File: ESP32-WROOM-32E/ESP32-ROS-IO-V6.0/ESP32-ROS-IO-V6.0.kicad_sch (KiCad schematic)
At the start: 2 parts, among them J1 Conn_01x22_Socket, J2 Conn_01x22_Socket

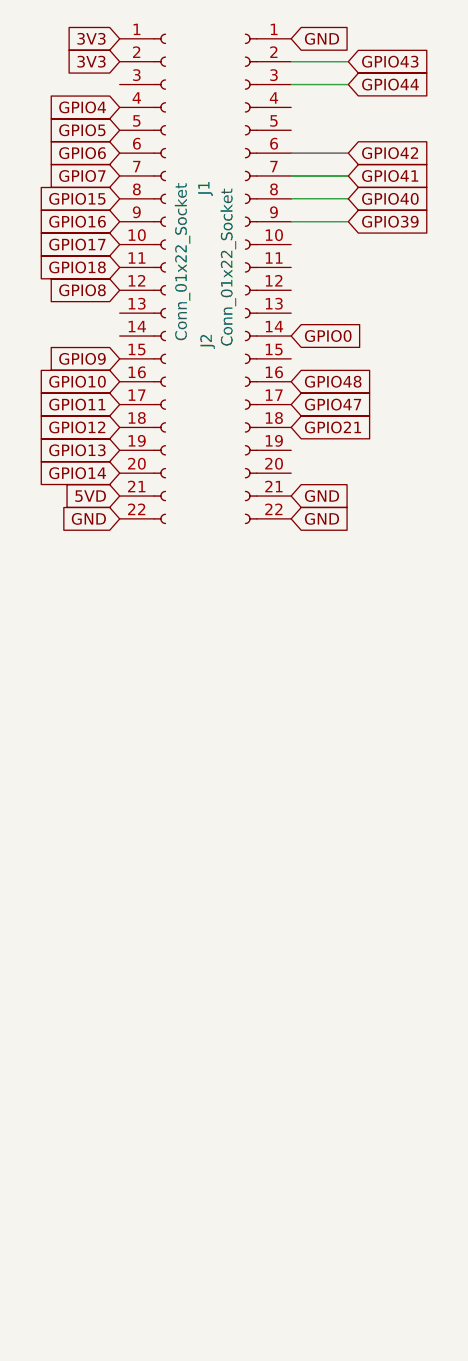
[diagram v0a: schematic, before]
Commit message: う
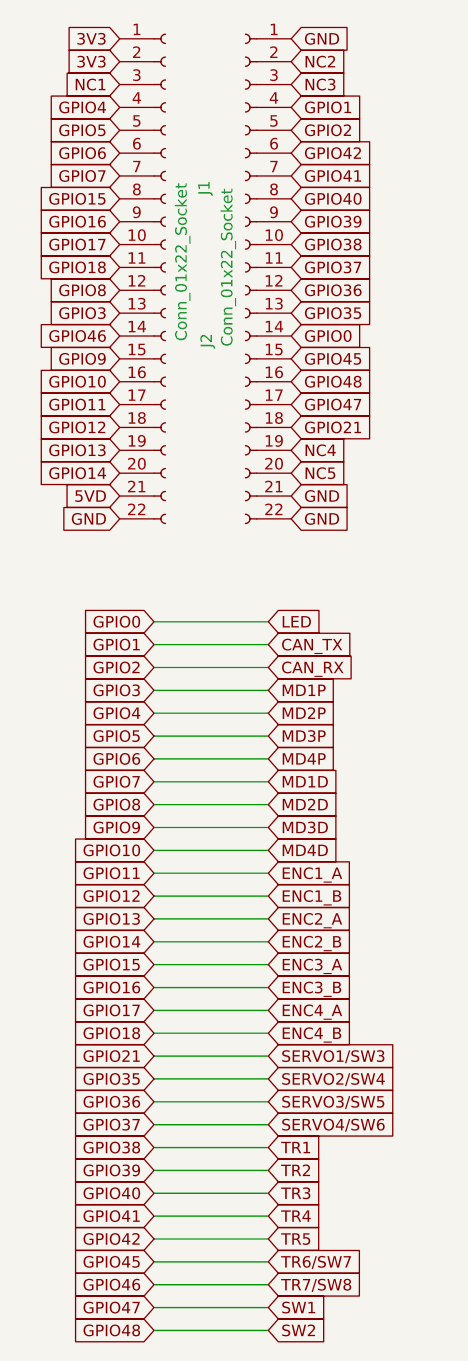
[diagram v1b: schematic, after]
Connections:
- net GPIO38: now reaches J2.10 (Pin_10)
- net GPIO37: now reaches J2.11 (Pin_11)
- net GPIO36: now reaches J2.12 (Pin_12)
- net GPIO35: now reaches J2.13 (Pin_13)
- net GPIO45: now reaches J2.15 (Pin_15)
- net NC4: now reaches J2.19 (Pin_19)
- net NC5: now reaches J2.20 (Pin_20)
- net CAN_TX: now reaches J2.4 (Pin_4)
- net CAN_RX: now reaches J2.5 (Pin_5)
- net GPIO3: now reaches J1.13 (Pin_13)
- net GPIO46: now reaches J1.14 (Pin_14)
- net NC1: now reaches J1.3 (Pin_3)
- net GPIO11 renamed ENC1_A
- net GPIO12 renamed ENC1_B
- net GPIO13 renamed ENC2_A
- net GPIO14 renamed ENC2_B
- net GPIO15 renamed ENC3_A
- net GPIO16 renamed ENC3_B
- net GPIO17 renamed ENC4_A
- net GPIO18 renamed ENC4_B
- net GPIO43 renamed NC2
- net GPIO44 renamed NC3

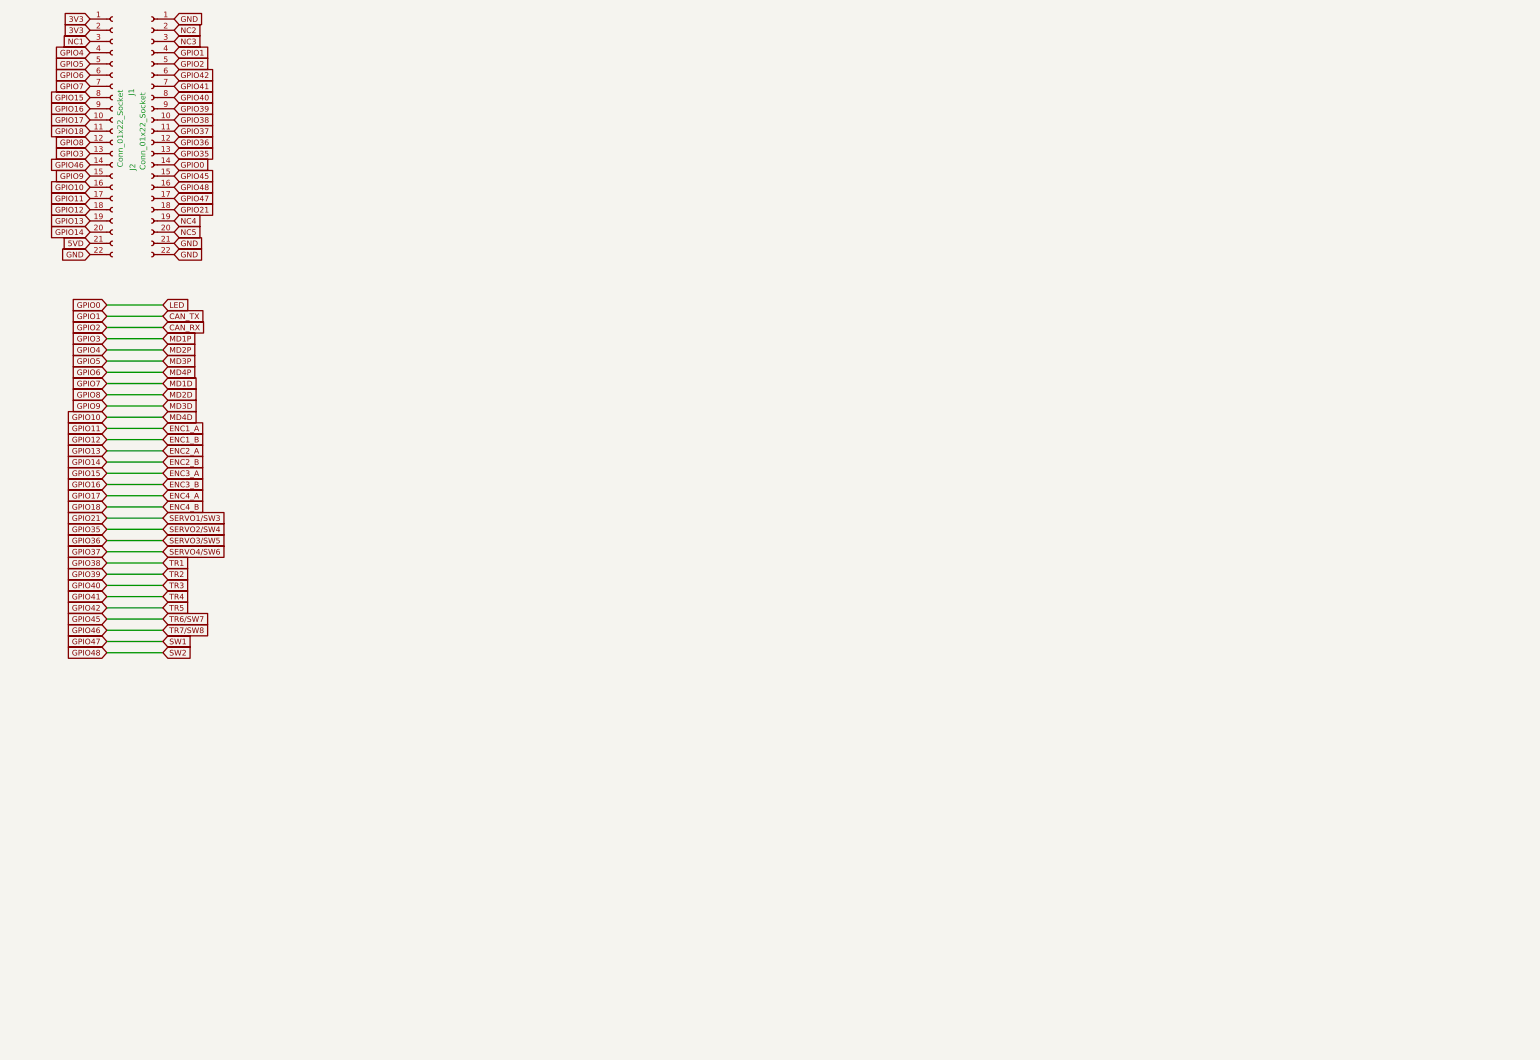
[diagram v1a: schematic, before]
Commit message: 回路図
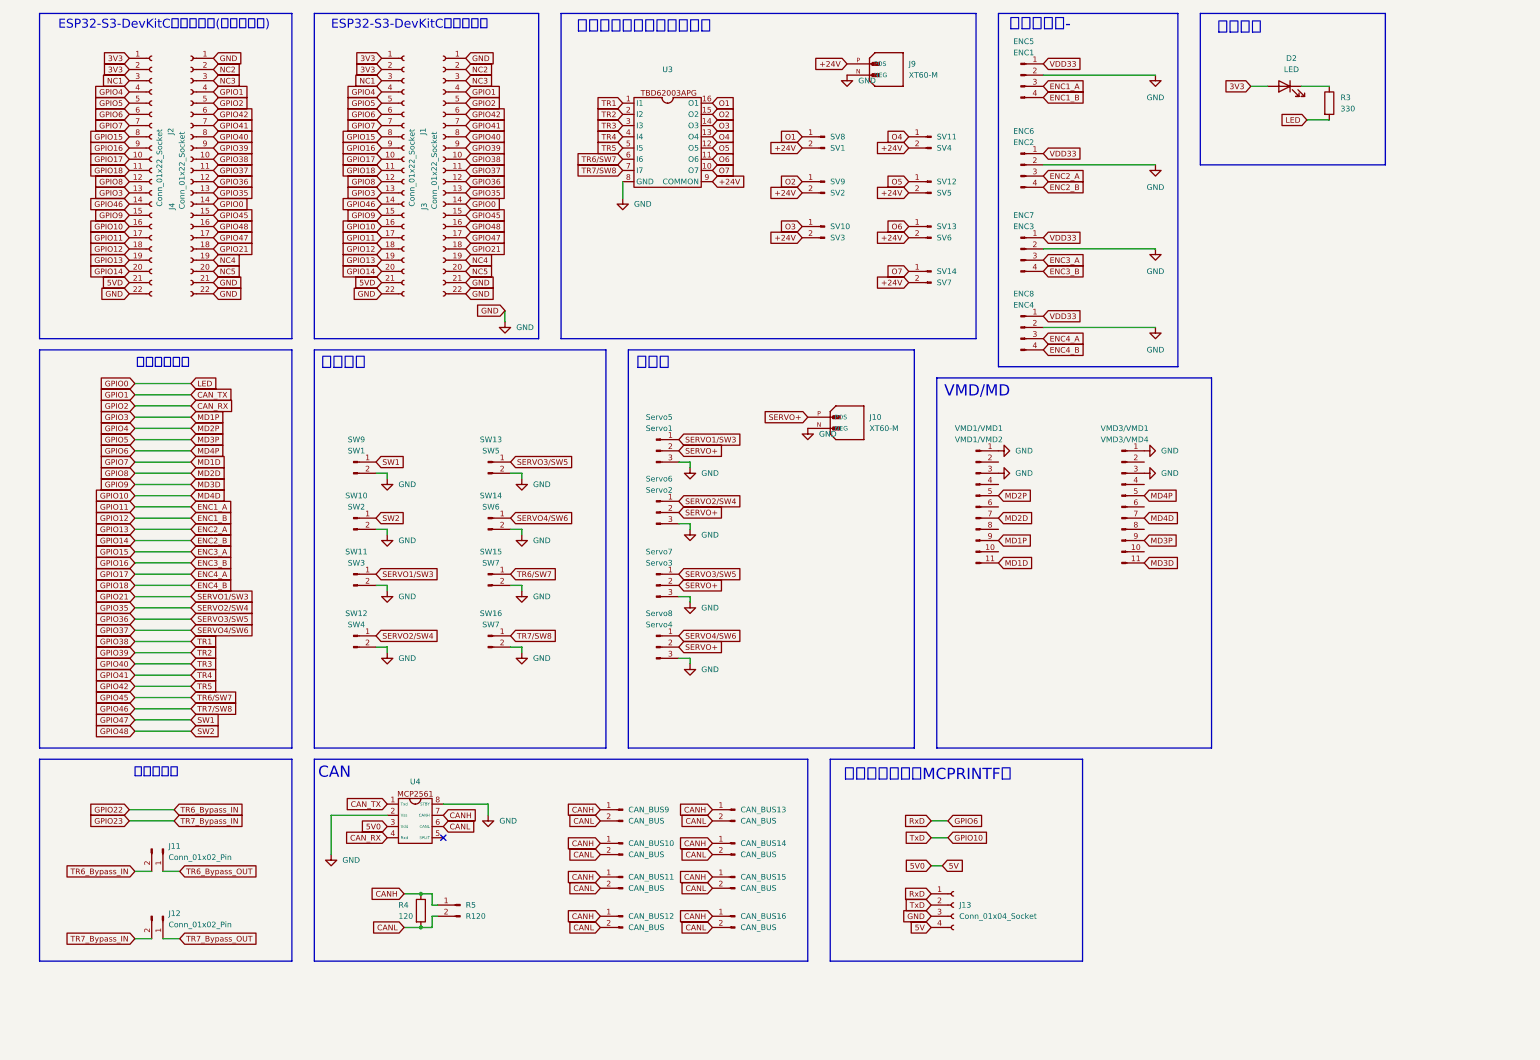
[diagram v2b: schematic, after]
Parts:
- added CAN_BUS10, CAN_BUS11, CAN_BUS12, CAN_BUS13, CAN_BUS14, CAN_BUS15, CAN_BUS16, CAN_BUS9: CAN_BUS, Connector_JST:JST_XH_B2B-XH-A_1x02_P2.50mm_Vertical, symbol Connector:Conn_01x02_Pin
- added D2: LED, LED_THT:LED_D5.0mm, symbol Device:LED
- added ENC5: ENC1, Connector_JST:JST_XH_B4B-XH-A_1x04_P2.50mm_Vertical, symbol Connector:Conn_01x04_Pin
- added ENC6: ENC2, Connector_JST:JST_XH_B4B-XH-A_1x04_P2.50mm_Vertical, symbol Connector:Conn_01x04_Pin
- added ENC7: ENC3, Connector_JST:JST_XH_B4B-XH-A_1x04_P2.50mm_Vertical, symbol Connector:Conn_01x04_Pin
- added ENC8: ENC4, Connector_JST:JST_XH_B4B-XH-A_1x04_P2.50mm_Vertical, symbol Connector:Conn_01x04_Pin
- added J1, J3: Conn_01x22_Socket, symbol Connector:Conn_01x22_Socket
- added J10, J9: XT60-M, XT60-M:AMASS_XT60-M, symbol XT60-M:XT60-M
- added J11, J12: Conn_01x02_Pin, Connector_PinHeader_2.54mm:PinHeader_1x02_P2.54mm_Vertical, symbol Connector:Conn_01x02_Pin
- added J13: Conn_01x04_Socket, Connector_PinSocket_2.54mm:PinSocket_1x04_P2.54mm_Vertical, symbol Connector:Conn_01x04_Socket
- added R3: 330, Resistor_THT:R_Axial_DIN0207_L6.3mm_D2.5mm_P10.16mm_Horizontal, symbol Device:R
- added R4: 120, Resistor_THT:R_Axial_DIN0207_L6.3mm_D2.5mm_P10.16mm_Horizontal, symbol Device:R
- added R5: R120, Connector_PinHeader_2.54mm:PinHeader_1x02_P2.54mm_Vertical, symbol Connector:Conn_01x02_Pin
- added SV10: SV3, Connector_JST:JST_XH_B2B-XH-A_1x02_P2.50mm_Vertical, symbol Connector:Conn_01x02_Pin
- added SV11: SV4, Connector_JST:JST_XH_B2B-XH-A_1x02_P2.50mm_Vertical, symbol Connector:Conn_01x02_Pin
- added SV12: SV5, Connector_JST:JST_XH_B2B-XH-A_1x02_P2.50mm_Vertical, symbol Connector:Conn_01x02_Pin
- added SV13: SV6, Connector_JST:JST_XH_B2B-XH-A_1x02_P2.50mm_Vertical, symbol Connector:Conn_01x02_Pin
- added SV14: SV7, Connector_JST:JST_XH_B2B-XH-A_1x02_P2.50mm_Vertical, symbol Connector:Conn_01x02_Pin
- added SV8: SV1, Connector_JST:JST_XH_B2B-XH-A_1x02_P2.50mm_Vertical, symbol Connector:Conn_01x02_Pin
- added SV9: SV2, Connector_JST:JST_XH_B2B-XH-A_1x02_P2.50mm_Vertical, symbol Connector:Conn_01x02_Pin
- added SW10: SW2, Connector_JST:JST_XH_B2B-XH-A_1x02_P2.50mm_Vertical, symbol Connector:Conn_01x02_Pin
- added SW11: SW3, Connector_JST:JST_XH_B2B-XH-A_1x02_P2.50mm_Vertical, symbol Connector:Conn_01x02_Pin
- added SW12: SW4, Connector_JST:JST_XH_B2B-XH-A_1x02_P2.50mm_Vertical, symbol Connector:Conn_01x02_Pin
- added SW13: SW5, Connector_JST:JST_XH_B2B-XH-A_1x02_P2.50mm_Vertical, symbol Connector:Conn_01x02_Pin
- added SW14: SW6, Connector_JST:JST_XH_B2B-XH-A_1x02_P2.50mm_Vertical, symbol Connector:Conn_01x02_Pin
- added SW15, SW16: SW7, Connector_JST:JST_XH_B2B-XH-A_1x02_P2.50mm_Vertical, symbol Connector:Conn_01x02_Pin
- added SW9: SW1, Connector_JST:JST_XH_B2B-XH-A_1x02_P2.50mm_Vertical, symbol Connector:Conn_01x02_Pin
- added Servo5: Servo1, Connector_JST:JST_XH_B3B-XH-A_1x03_P2.50mm_Vertical, symbol Connector:Conn_01x03_Pin
- added Servo6: Servo2, Connector_JST:JST_XH_B3B-XH-A_1x03_P2.50mm_Vertical, symbol Connector:Conn_01x03_Pin
- added Servo7: Servo3, Connector_JST:JST_XH_B3B-XH-A_1x03_P2.50mm_Vertical, symbol Connector:Conn_01x03_Pin
- added Servo8: Servo4, Connector_JST:JST_XH_B3B-XH-A_1x03_P2.50mm_Vertical, symbol Connector:Conn_01x03_Pin
- added U3: ~, Package_DIP:DIP-16_W7.62mm, symbol New_Library:TBD62003APG
- added U4: ~, Package_DIP:DIP-8_W7.62mm, symbol New_Library:MCP2561
- added VMD1/VMD1: VMD1/VMD2, Connector_PinHeader_2.54mm:PinHeader_1x11_P2.54mm_Vertical, symbol Connector:Conn_01x11_Pin
- added VMD3/VMD1: VMD3/VMD4, Connector_PinHeader_2.54mm:PinHeader_1x11_P2.54mm_Vertical, symbol Connector:Conn_01x11_Pin
- renumbered J1 to J2, J2 to J4
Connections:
- net 3V3: now also D2.2 (A), J1.1 (Pin_1), J1.2 (Pin_2)
- net 5VD: now also J1.21 (Pin_21)
- net CAN_RX: now also J3.5 (Pin_5), U4.4 (Rxd)
- net CAN_TX: now also J3.4 (Pin_4), U4.1 (Txd)
- net ENC1_A: now also ENC5.3 (Pin_3), J1.17 (Pin_17)
- net ENC1_B: now also ENC5.4 (Pin_4), J1.18 (Pin_18)
- net ENC2_A: now also ENC6.3 (Pin_3), J1.19 (Pin_19)
- net ENC2_B: now also ENC6.4 (Pin_4), J1.20 (Pin_20)
- net ENC3_A: now also ENC7.3 (Pin_3), J1.8 (Pin_8)
- net ENC3_B: now also ENC7.4 (Pin_4), J1.9 (Pin_9)
- net ENC4_A: now also ENC8.3 (Pin_3), J1.10 (Pin_10)
- net ENC4_B: now also ENC8.4 (Pin_4), J1.11 (Pin_11)
- net GND: now also ENC5.2 (Pin_2), ENC6.2 (Pin_2), ENC7.2 (Pin_2), ENC8.2 (Pin_2), J1.22 (Pin_22), J10.N (NEG), J13.3 (Pin_3), J3.1 (Pin_1), J3.21 (Pin_21), J3.22 (Pin_22), J9.N (NEG), SW10.2 (Pin_2), SW11.2 (Pin_2), SW12.2 (Pin_2), SW13.2 (Pin_2), SW14.2 (Pin_2), SW15.2 (Pin_2), SW16.2 (Pin_2), SW9.2 (Pin_2), Servo5.3 (Pin_3), Servo6.3 (Pin_3), Servo7.3 (Pin_3), Servo8.3 (Pin_3), U3.8 (GND), U4.2 (Vss), U4.8 (STBY), VMD1/VMD1.1 (Pin_1), VMD1/VMD1.3 (Pin_3), VMD3/VMD1.1 (Pin_1), VMD3/VMD1.3 (Pin_3)
- net GPIO0: now also J3.14 (Pin_14), R3.2
- net GPIO10: now also J1.16 (Pin_16), J13.2 (Pin_2), VMD3/VMD1.7 (Pin_7)
- net GPIO21: now also J3.18 (Pin_18), SW11.1 (Pin_1), Servo5.1 (Pin_1)
- net GPIO3: now also J1.13 (Pin_13), VMD1/VMD1.9 (Pin_9)
- net GPIO35: now also J3.13 (Pin_13), SW12.1 (Pin_1), Servo6.1 (Pin_1)
- net GPIO36: now also J3.12 (Pin_12), SW13.1 (Pin_1), Servo7.1 (Pin_1)
- net GPIO37: now also J3.11 (Pin_11), SW14.1 (Pin_1), Servo8.1 (Pin_1)
- net GPIO38: now also J3.10 (Pin_10), U3.1 (I1)
- net GPIO39: now also J3.9 (Pin_9), U3.2 (I2)
- net GPIO4: now also J1.4 (Pin_4), VMD1/VMD1.5 (Pin_5)
- net GPIO40: now also J3.8 (Pin_8), U3.3 (I3)
- net GPIO41: now also J3.7 (Pin_7), U3.4 (I4)
- net GPIO42: now also J3.6 (Pin_6), U3.5 (I5)
- net GPIO45: now also J3.15 (Pin_15), SW15.1 (Pin_1), U3.6 (I6)
- net GPIO46: now also J1.14 (Pin_14), SW16.1 (Pin_1), U3.7 (I7)
- net GPIO47: now also J3.17 (Pin_17), SW9.1 (Pin_1)
- net GPIO48: now also J3.16 (Pin_16), SW10.1 (Pin_1)
- net GPIO5: now also J1.5 (Pin_5), VMD3/VMD1.9 (Pin_9)
- net GPIO6: now also J1.6 (Pin_6), J13.1 (Pin_1), VMD3/VMD1.5 (Pin_5)
- net GPIO7: now also J1.7 (Pin_7), VMD1/VMD1.11 (Pin_11)
- net GPIO8: now also J1.12 (Pin_12), VMD1/VMD1.7 (Pin_7)
- net GPIO9: now also J1.15 (Pin_15), VMD3/VMD1.11 (Pin_11)
- net NC1: now also J1.3 (Pin_3)
- net NC2: now also J3.2 (Pin_2)
- net NC3: now also J3.3 (Pin_3)
- net NC4: now also J3.19 (Pin_19)
- net NC5: now also J3.20 (Pin_20)
- new net: D2.1 (K), R3.1
- new net +24V: J9.P (POS), SV10.2 (Pin_2), SV11.2 (Pin_2), SV12.2 (Pin_2), SV13.2 (Pin_2), SV14.2 (Pin_2), SV8.2 (Pin_2), SV9.2 (Pin_2), U3.9 (COMMON)
- new net 5V: J13.4 (Pin_4), U4.3 (Vdd)
- new net CANH: CAN_BUS10.1 (Pin_1), CAN_BUS11.1 (Pin_1), CAN_BUS12.1 (Pin_1), CAN_BUS13.1 (Pin_1), CAN_BUS14.1 (Pin_1), CAN_BUS15.1 (Pin_1), CAN_BUS16.1 (Pin_1), CAN_BUS9.1 (Pin_1), R4.1, R5.1 (Pin_1), U4.7 (CANH)
- new net CANL: CAN_BUS10.2 (Pin_2), CAN_BUS11.2 (Pin_2), CAN_BUS12.2 (Pin_2), CAN_BUS13.2 (Pin_2), CAN_BUS14.2 (Pin_2), CAN_BUS15.2 (Pin_2), CAN_BUS16.2 (Pin_2), CAN_BUS9.2 (Pin_2), R4.2, R5.2 (Pin_2), U4.6 (CANL)
- new net GPIO22: J11.2 (Pin_2)
- new net GPIO23: J12.2 (Pin_2)
- new net O1: SV8.1 (Pin_1), U3.16 (O1)
- new net O2: SV9.1 (Pin_1), U3.15 (O2)
- new net O3: SV10.1 (Pin_1), U3.14 (O3)
- new net O4: SV11.1 (Pin_1), U3.13 (O4)
- new net O5: SV12.1 (Pin_1), U3.12 (O5)
- new net O6: SV13.1 (Pin_1), U3.11 (O6)
- new net O7: SV14.1 (Pin_1), U3.10 (O7)
- new net SERVO+: J10.P (POS), Servo5.2 (Pin_2), Servo6.2 (Pin_2), Servo7.2 (Pin_2), Servo8.2 (Pin_2)
- new net TR6_Bypass_OUT: J11.1 (Pin_1)
- new net TR7_Bypass_OUT: J12.1 (Pin_1)
- new net VDD33: ENC5.1 (Pin_1), ENC6.1 (Pin_1), ENC7.1 (Pin_1), ENC8.1 (Pin_1)
- no-connect marks 0 -> 1
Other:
- note added: "CAN"
- note added: "ESP32-S3-DevKitC用ソケット"
- note added: "ESP32-S3-DevKitC用ソケット(デバッグ用)"
- note added: "VMD/MD"
- note added: "エンコーダ-"
- note added: "サーボ"
- note added: "スイッチ"
- note added: "ソレノイドバルブ・表示灯"
- note added: "バイパス用"
- note added: "ピン割り当て"
- note added: "外部シリアル（MCPRINTF）"
- note added: "状態表示"
- moved on the sheet: J2, J4

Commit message: 回路図変更
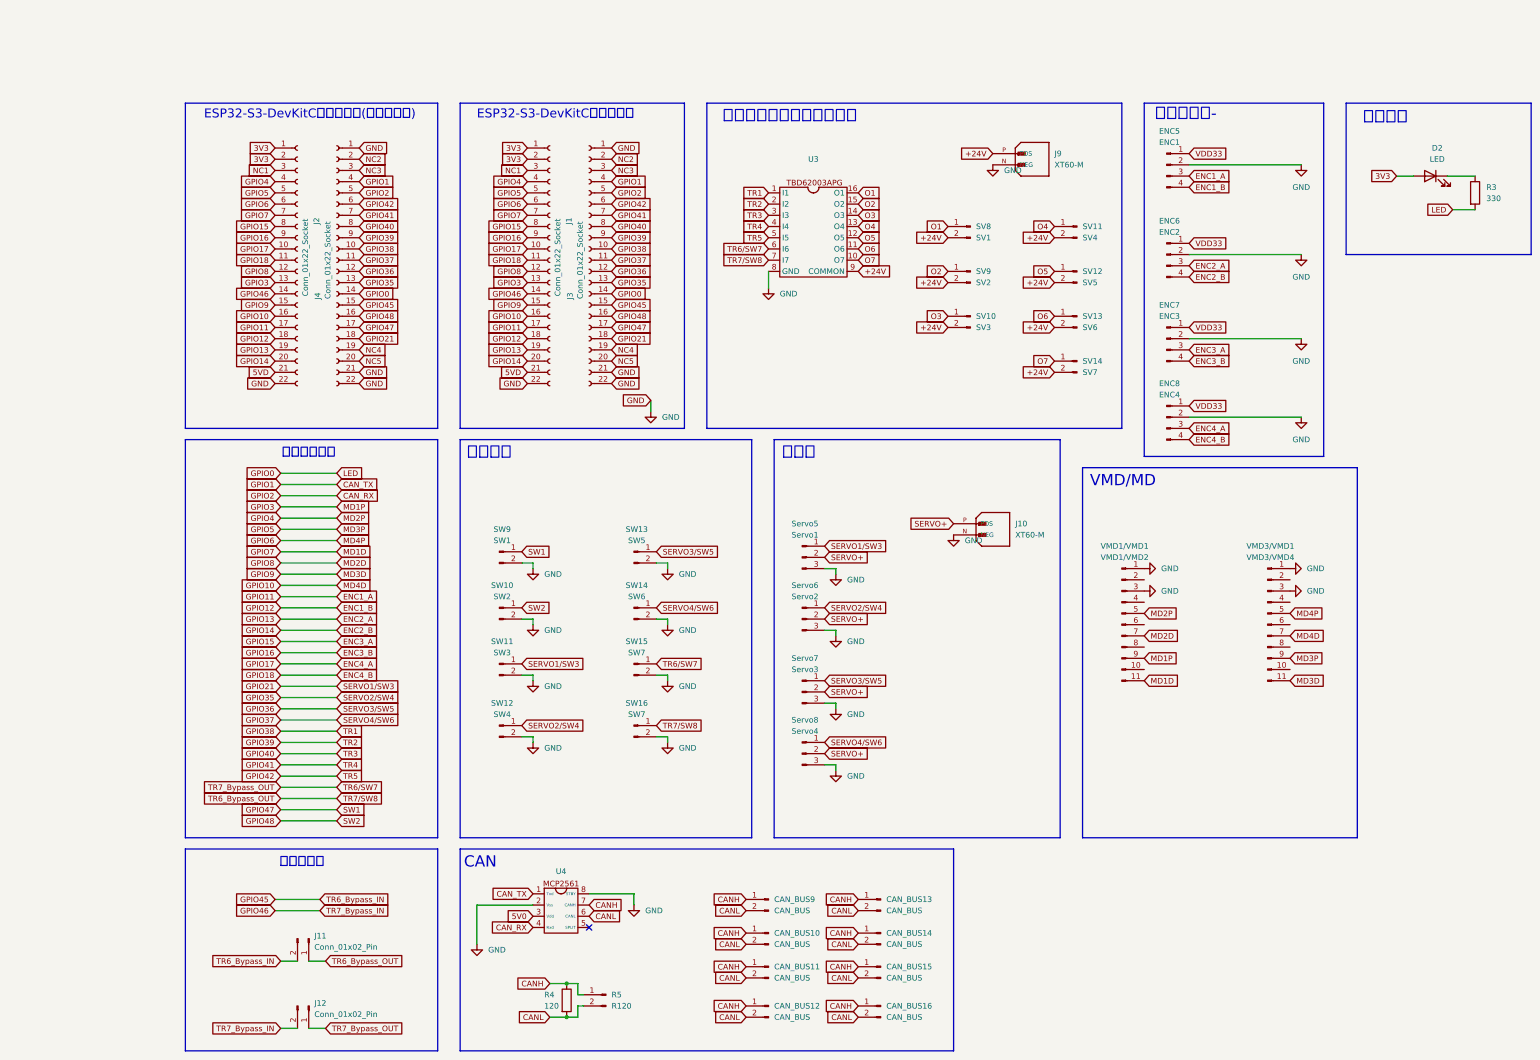
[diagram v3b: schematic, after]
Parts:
- removed J13: Conn_01x04_Socket, Connector_PinSocket_2.54mm:PinSocket_1x04_P2.54mm_Vertical, symbol Connector:Conn_01x04_Socket
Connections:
- net GPIO22 is gone; now on net GPIO45: J11.2 (Pin_2)
- net GPIO23 is gone; now on net GPIO46: J12.2 (Pin_2)
- net GPIO45: no longer SW15.1 (Pin_1), U3.6 (I6)
- net GPIO46: no longer SW16.1 (Pin_1), U3.7 (I7)
- net TR6_Bypass_OUT: now also SW16.1 (Pin_1), U3.7 (I7)
- net 5V renamed 5V0
- net TR7_Bypass_OUT renamed TR6/SW7
- net TR6/SW7: now also SW15.1 (Pin_1), U3.6 (I6)
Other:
- note removed: "外部シリアル（MCPRINTF）"
- moved on the sheet: CAN_BUS10, CAN_BUS11, CAN_BUS12, CAN_BUS13, CAN_BUS14, CAN_BUS15, CAN_BUS16, CAN_BUS9, D2, ENC5, ENC6, ENC7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
